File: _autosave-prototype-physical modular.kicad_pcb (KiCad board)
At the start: 2 copper layers, 100 x 164 mm, 177 parts, among them CON1 BARREL_JACK, CON2 SD_Card, IC1 ATMEGA2560-A, J1 MIDI_IN, J2 MIDI_OUT, P1 POWER, P13 PD, P15 PH, P16 PF, P17 SD_PINS, P18 3VI2C, P19 PIGPIO, P2 FTDI, P3 SPI, P4 BUSTI, P5 BUSTO, P7 PA, P9 PB, Q1 BSS138, Q2 BSS138, Q3 BSS138, Q4 BSS138, Q5 BSS138, Q6 BSS138, SW1 SW_PUSH, SW10 SW_PUSH, SW11 SW_PUSH, SW12 SW_PUSH, SW13 SW_PUSH, SW14 SW_PUSH, SW2 ROTARY_ENCODER_SWITCH, SW3 SW_PUSH, SW4 SW_PUSH, SW5 SW_PUSH, SW6 SW_PUSH, SW7 SW_PUSH, SW8 SW_PUSH, SW9 SW_PUSH, U1 NCP1117ST50T3G, U2 6N138, Y1 16MHz

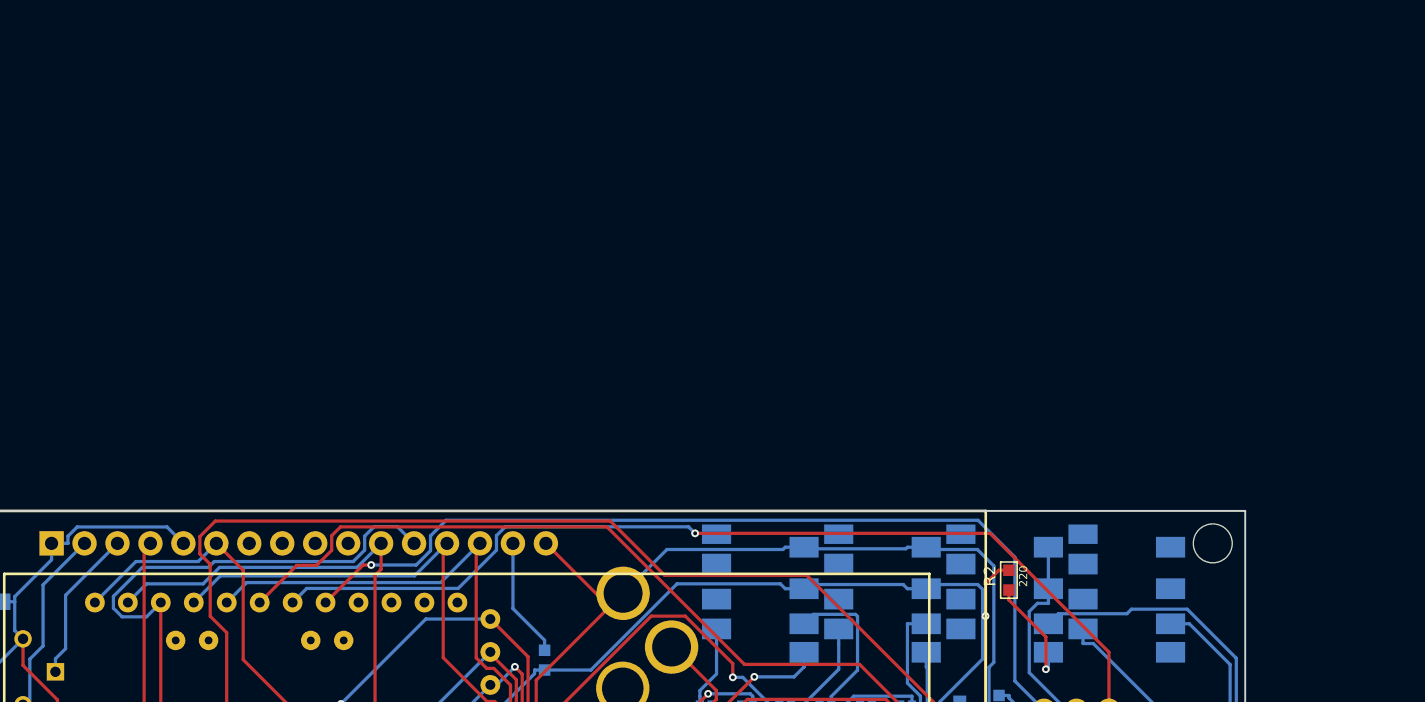
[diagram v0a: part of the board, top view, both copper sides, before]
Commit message: update gerbers
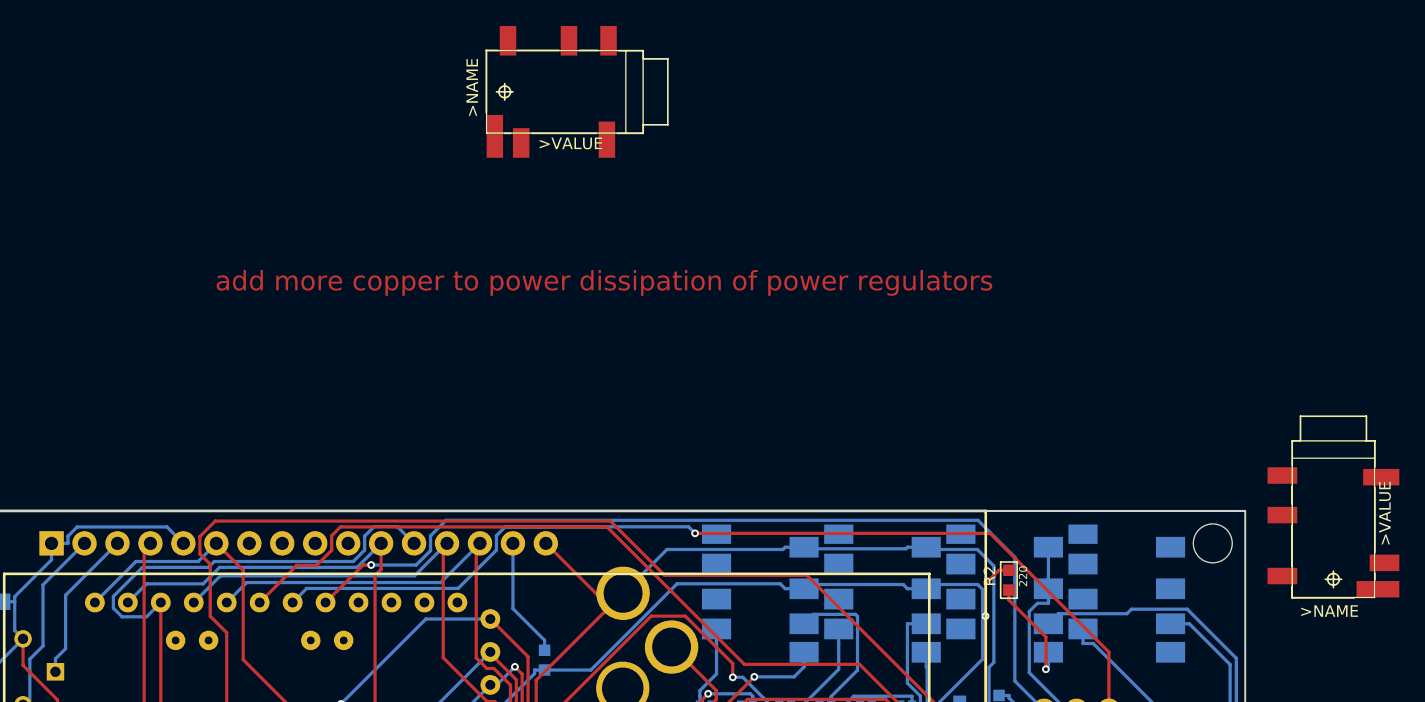
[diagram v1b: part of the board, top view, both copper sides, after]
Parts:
- added >NAME: >VALUE, SeeedOPL-Connector:AUDIO6P-SMD-3.5-14.0X6.4X5.0MM, F.Cu at (106.8, -7.30)
- added >NAME: >VALUE, SeeedOPL-Connector:AUDIO6P-SMD-3.5-14.0X6.4X5.0MM, F.Cu at (55.5, -32.3)
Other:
- board text added: "add more copper to power dissipation of power regulators"
